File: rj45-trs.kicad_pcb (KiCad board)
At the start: 2 copper layers, 50 x 38 mm, 5 parts, among them J101 NSJ12HC, J102 NSJ12HC, J103 NE8FAH

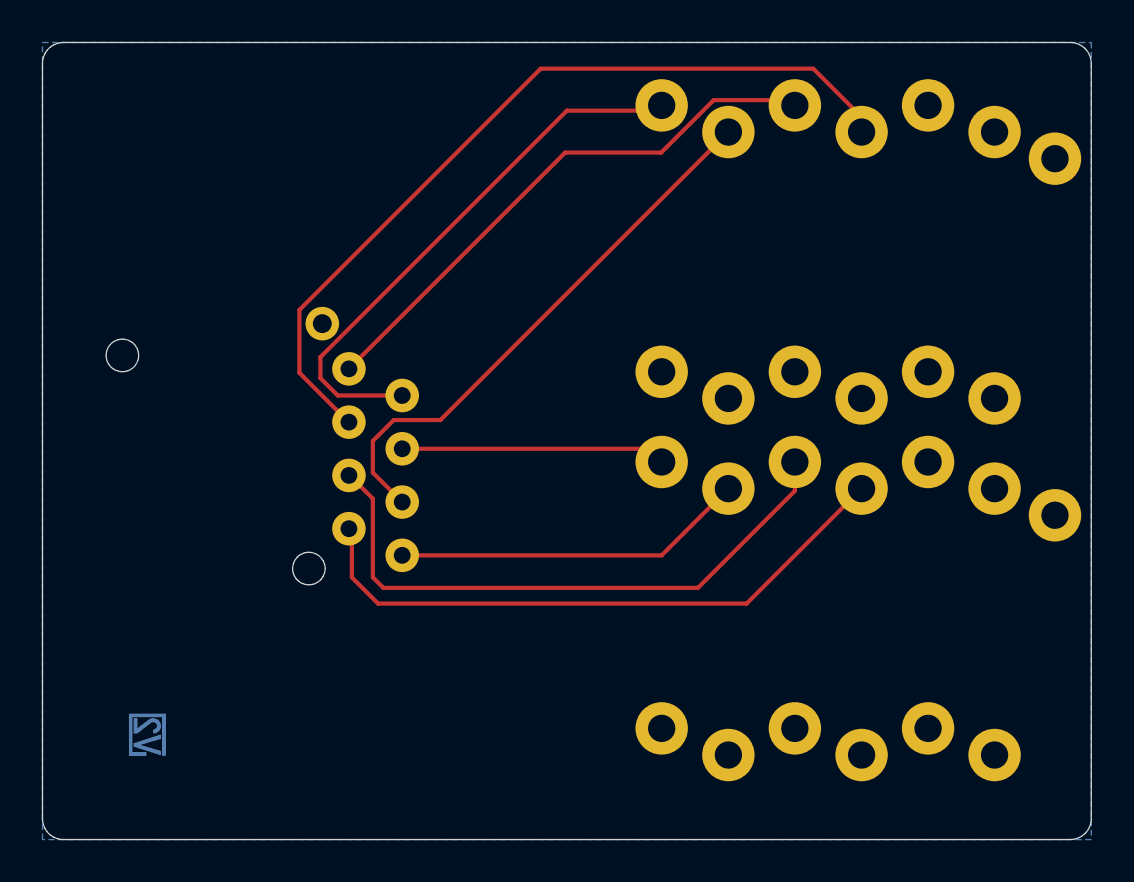
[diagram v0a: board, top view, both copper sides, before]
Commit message: Update
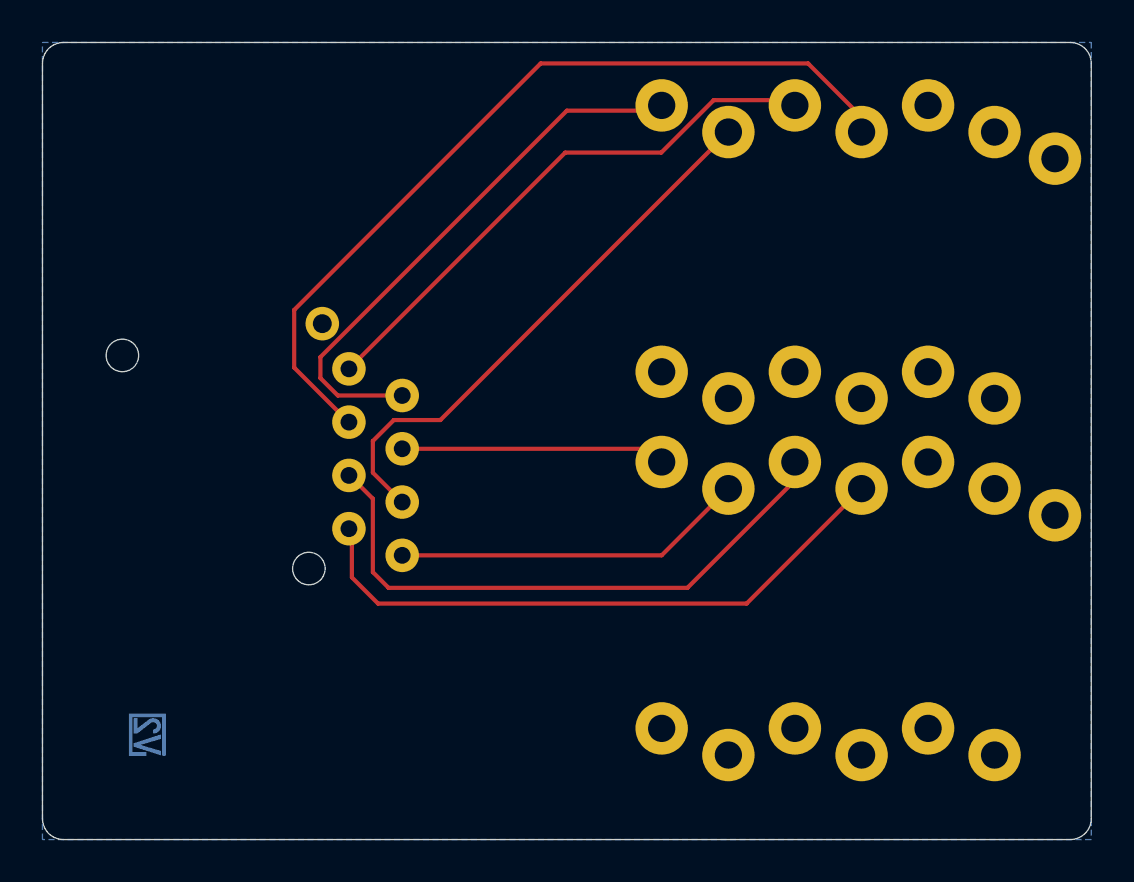
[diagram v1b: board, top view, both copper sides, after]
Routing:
- net /Channel-3-: track 39.6 -> 40.1 mm
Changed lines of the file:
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@@
 	)
 	(segment
-		(start 86.25 79.957107)
-		(end 99.25 79.957107)
-		(width 0.2)
-		(layer "F.Cu")
-		(net 2)
-	)
-	(segment
-		(start 77.1 96.807107)
-		(end 74.75 94.457107)
+		(start 74.5 94.207107)
+		(end 74.5 91.457107)
 		(width 0.2)
 		(layer "F.Cu")
@@
 	)
 	(segment
-		(start 74.75 91.457107)
-		(end 86.25 79.957107)
-		(width 0.2)
-		(layer "F.Cu")
-		(net 2)
-	)
-	(segment
-		(start 99.25 79.957107)
-		(end 101.5 82.207107)
+		(start 101.5 82.927107)
+		(end 101.55 82.977107)
+		(width 0.2)
+		(layer "F.Cu")
+		(net 2)
+	)
+	(segment
+		(start 74.5 91.457107)
+		(end 86.25 79.707107)
 		(width 0.2)
 		(layer "F.Cu")
@@
 	)
 	(segment
-		(start 74.75 94.457107)
-		(end 74.75 91.457107)
-		(width 0.2)
-		(layer "F.Cu")
-		(net 2)
-	)
-	(segment
-		(start 101.5 82.927107)
-		(end 101.55 82.977107)
+		(start 99 79.707107)
+		(end 101.5 82.207107)
+		(width 0.2)
+		(layer "F.Cu")
+		(net 2)
+	)
+	(segment
+		(start 77.1 96.807107)
+		(end 74.5 94.207107)
+		(width 0.2)
+		(layer "F.Cu")
+		(net 2)
+	)
+	(segment
+		(start 86.25 79.707107)
+		(end 99 79.707107)
 		(width 0.2)
 		(layer "F.Cu")
@@
 	)
 	(segment
+		(start 95.2 82.977107)
+		(end 81.47 96.707107)
+		(width 0.2)
+		(layer "F.Cu")
+		(net 4)
+	)
+	(segment
+		(start 78.25 97.707107)
+		(end 78.25 99.217107)
+		(width 0.2)
+		(layer "F.Cu")
+		(net 4)
+	)
+	(segment
 		(start 79.25 96.707107)
 		(end 78.25 97.707107)
@@
 	)
 	(segment
-		(start 95.2 82.977107)
-		(end 81.47 96.707107)
-		(width 0.2)
-		(layer "F.Cu")
-		(net 4)
-	)
-	(segment
-		(start 78.25 97.707107)
-		(end 78.25 99.217107)
-		(width 0.2)
-		(layer "F.Cu")
-		(net 4)
-	)
-	(segment
 		(start 77.25 104.207107)
 		(end 78.5 105.457107)
@@
 	)
 	(segment
-		(start 78.25 104.207107)
+		(start 78.25 100.457107)
+		(end 77.14 99.347107)
+		(width 0.2)
+		(layer "F.Cu")
+		(net 17)
+	)
+	(segment
+		(start 98.37 99.587107)
+		(end 93.25 104.707107)
+		(width 0.2)
+		(layer "F.Cu")
+		(net 17)
+	)
+	(segment
+		(start 79 104.707107)
+		(end 78.25 103.957107)
+		(width 0.2)
+		(layer "F.Cu")
+		(net 17)
+	)
+	(segment
+		(start 78.25 103.957107)
 		(end 78.25 100.457107)
+		(width 0.2)
+		(layer "F.Cu")
+		(net 17)
+	)
+	(segment
+		(start 98.37 98.707107)
+		(end 98.37 99.587107)
 		(width 0.2)
 		(layer "F.Cu")
@@
 	)
 	(segment
-		(start 78.25 100.457107)
-		(end 77.14 99.347107)
-		(width 0.2)
-		(layer "F.Cu")
-		(net 17)
-	)
-	(segment
-		(start 93.75 104.707107)
-		(end 78.75 104.707107)
-		(width 0.2)
-		(layer "F.Cu")
-		(net 17)
-	)
-	(segment
-		(start 78.75 104.707107)
-		(end 78.25 104.207107)
-		(width 0.2)
-		(layer "F.Cu")
-		(net 17)
-	)
-	(segment
-		(start 98.37 98.707107)
-		(end 98.37 100.087107)
-		(width 0.2)
-		(layer "F.Cu")
-		(net 17)
-	)
-	(segment
-		(start 98.37 100.087107)
-		(end 93.75 104.707107)
-		(width 0.2)
-		(layer "F.Cu")
+		(start 93.25 104.707107)
+		(end 79 104.707107)
+		(width 0.2)
+		(layer "F.Cu")

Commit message: Refresh
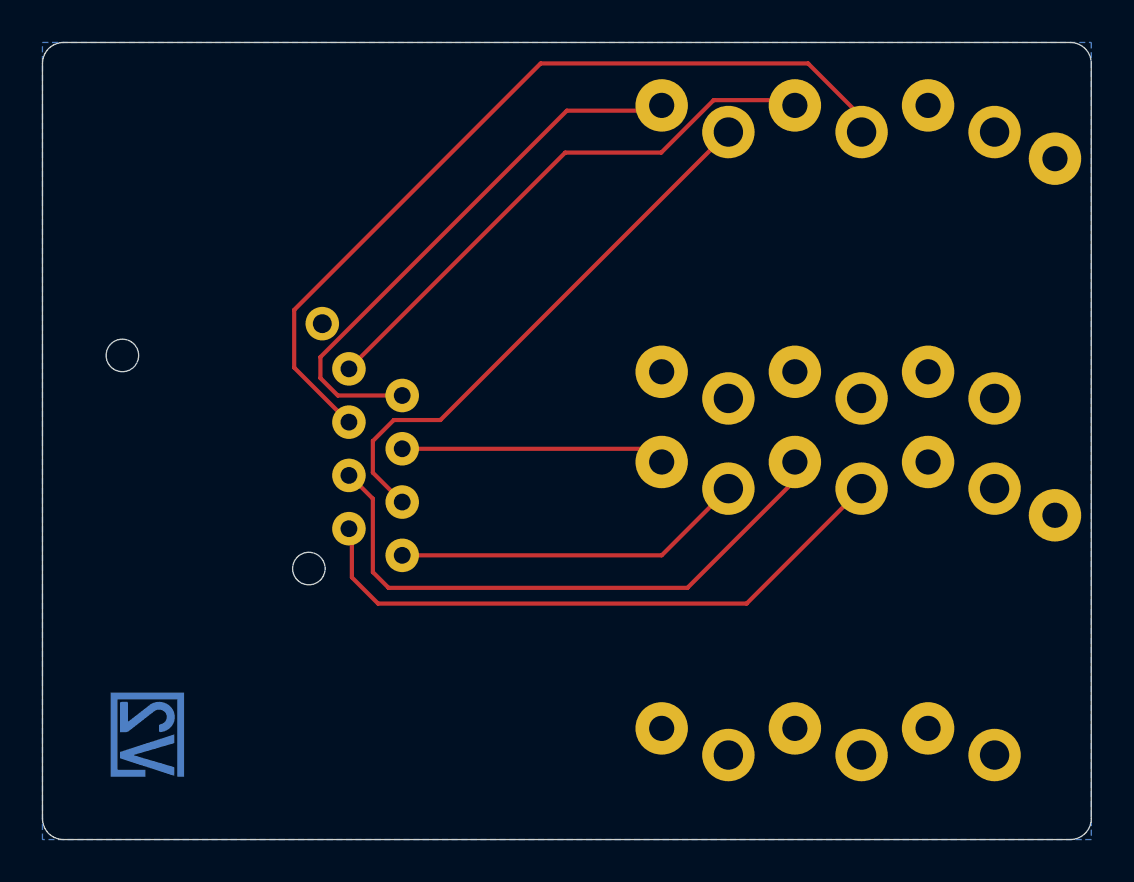
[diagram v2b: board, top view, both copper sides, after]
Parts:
- ICON101: footprint V2_Artwork:Logo_Tiny -> V2_Artwork:Logo_Small
